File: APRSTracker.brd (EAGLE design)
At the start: 100 x 80 mm, 32 parts, among them IC2 TP4056, X1 POWERSUPPLY_DC21MMX

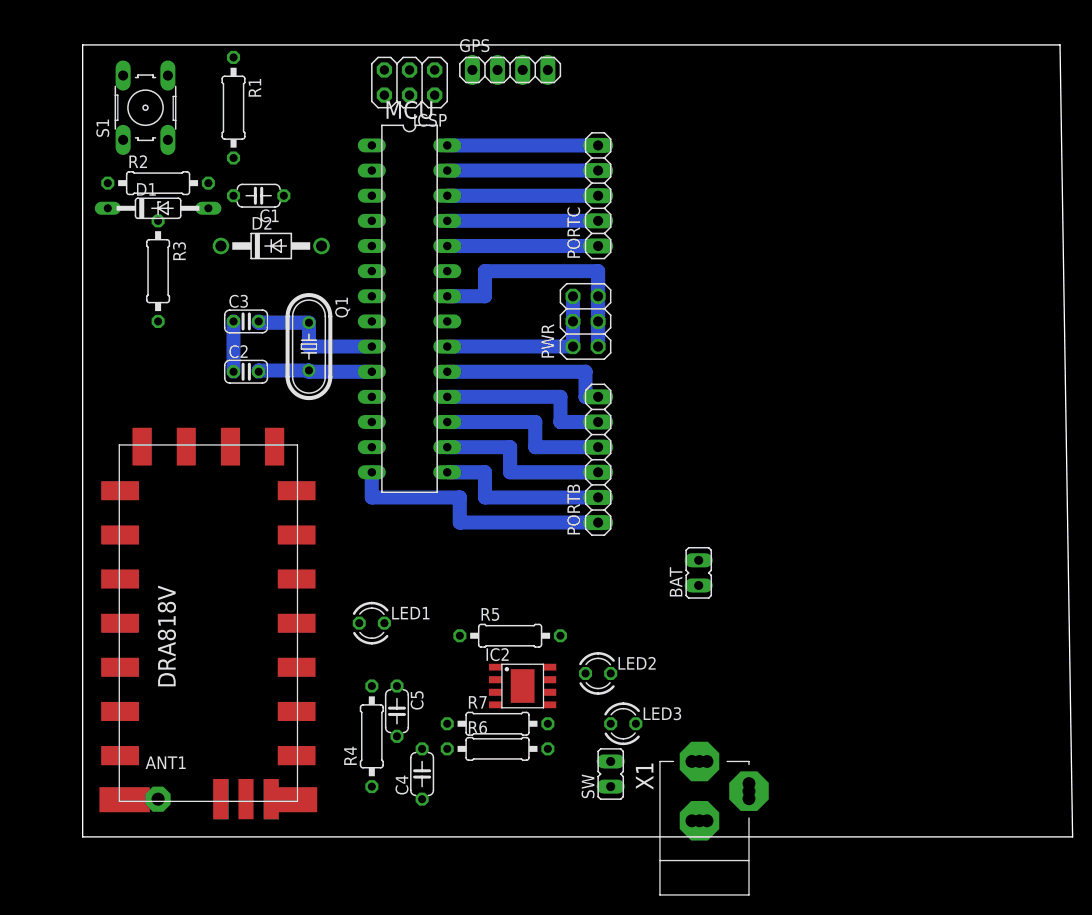
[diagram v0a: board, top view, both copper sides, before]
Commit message: brd v1
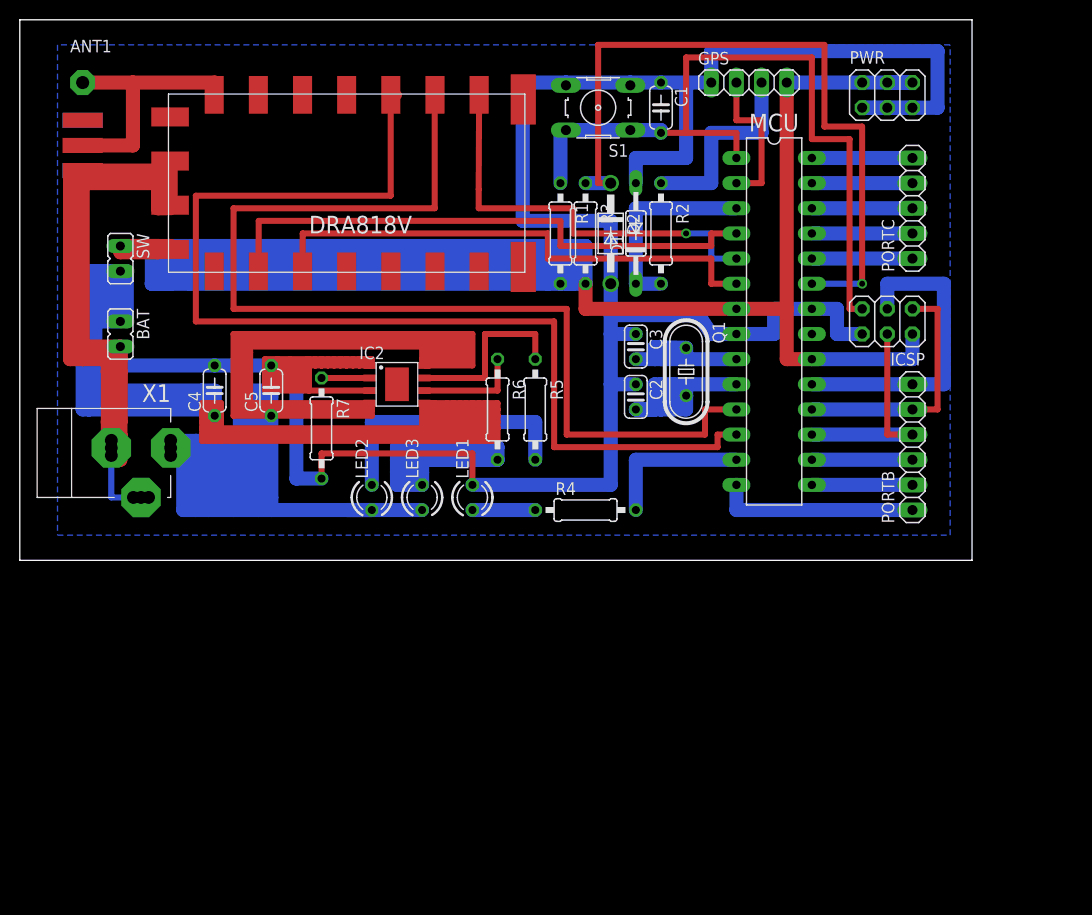
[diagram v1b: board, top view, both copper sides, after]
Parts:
- moved ANT1 72.8 mm to (0.00, 76.2)
- moved SW 71.9 mm to (3.81, 58.4), turned to 180 degrees
- moved X1 70.8 mm to (2.54, 39.4), turned to 90 degrees
- moved ANT 65.0 mm to (0.00, 67.3), turned to 90 degrees
- moved BAT 63.2 mm to (3.81, 50.8), turned to 180 degrees
- moved ICSP 54.0 mm to (81.3, 52.1)
- moved R2 51.1 mm to (58.4, 61.0), turned to 270 degrees
- moved D1 48.3 mm to (55.9, 61.0), turned to 90 degrees
- moved DRA818V 46.6 mm to (26.7, 66.0), turned to 180 degrees
- moved S1 45.7 mm to (52.1, 73.7), turned to 180 degrees
- moved C4 44.0 mm to (13.3, 45.1)
- moved R3 43.3 mm to (50.8, 61.0)
- moved C1 41.6 mm to (58.4, 73.7), turned to 270 degrees
- moved C2 39.5 mm to (55.9, 44.5), turned to 270 degrees
- moved C3 39.5 mm to (55.9, 49.5), turned to 270 degrees
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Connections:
- net GND: now also LED1.K; no longer R4.1
- net LED: now also R4.2; no longer LED1.A
- net N$3: now also LED1.A, R4.1; no longer LED1.K, R4.2
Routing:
- net GND: track 30.5 -> 431.6 mm
- net VCC: track 17.8 -> 392.1 mm
- net V-BAT: track 0.00 -> 367.6 mm
- net CHG: track 0.00 -> 308.9 mm, vias 0 -> 1
- net RF-RX: track 0.00 -> 112.4 mm
- net RF-TX: track 0.00 -> 108.0 mm
- net RESET: track 0.00 -> 76.8 mm
- net VD: track 0.00 -> 73.7 mm, vias 0 -> 1
- net PD2: track 0.00 -> 57.2 mm
- net PD4: track 0.00 -> 52.8 mm
- net N$7: track 0.00 -> 44.4 mm
- net PD3: track 0.00 -> 42.6 mm, vias 0 -> 1
- net N$4: track 0.00 -> 26.7 mm
- net N$1: track 0.00 -> 26.0 mm
- net N$6: track 11.7 -> 33.5 mm
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- added copper zone on layer 16, net GND
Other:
- board size 100 x 80 mm -> 96.2 x 54.6 mm
